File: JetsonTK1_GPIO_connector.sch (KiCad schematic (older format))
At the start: 3 parts

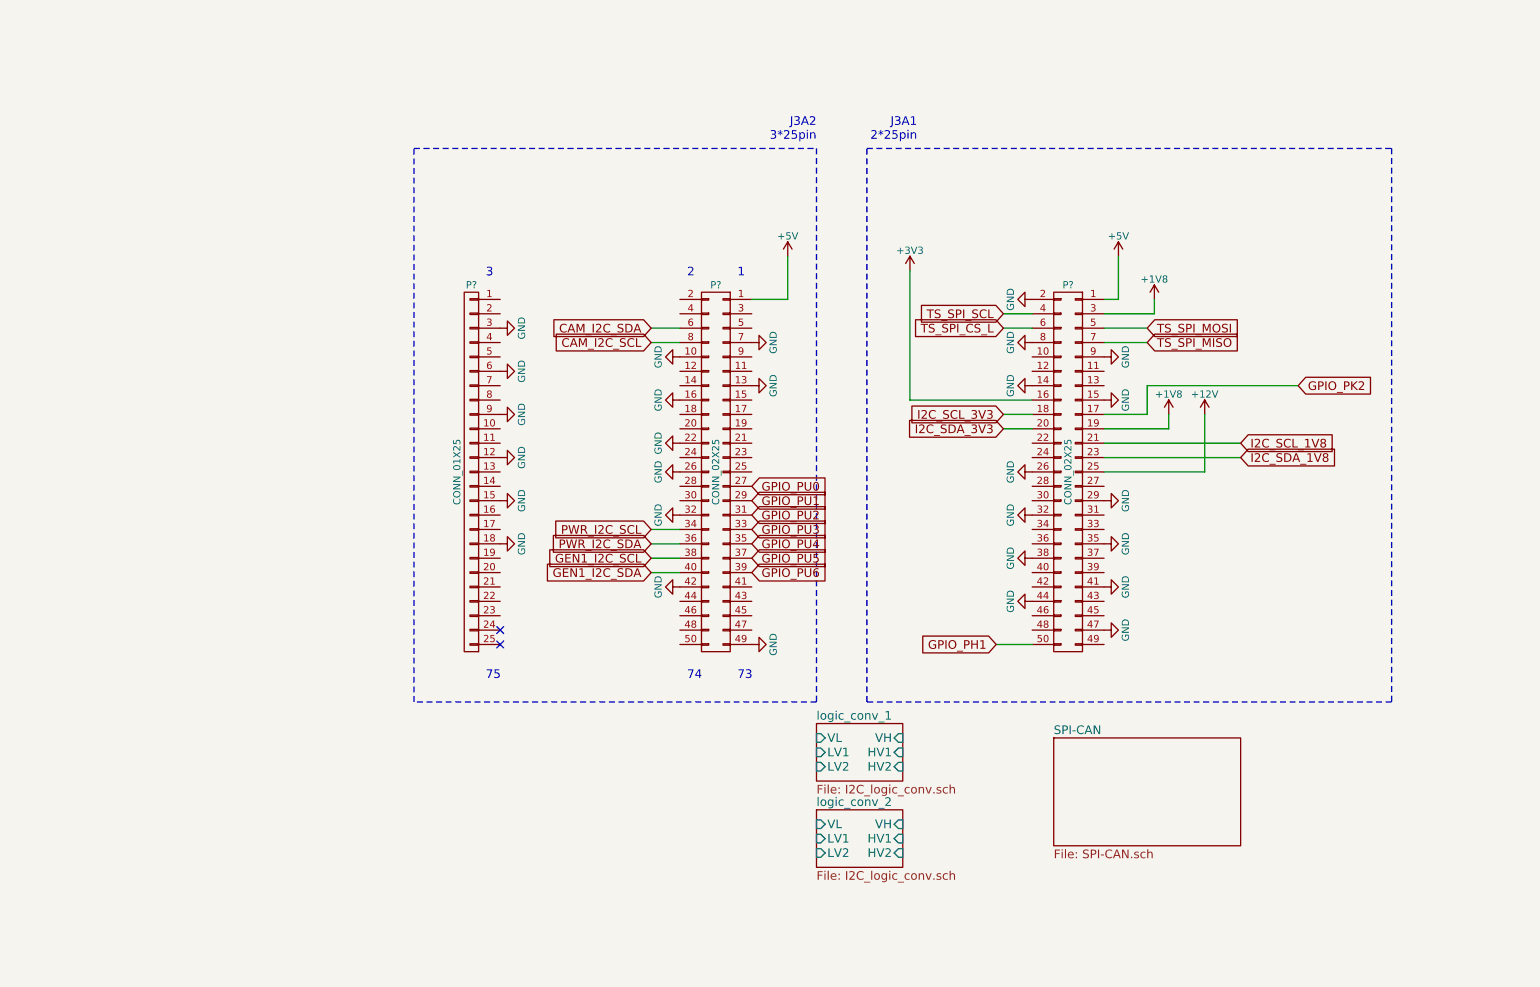
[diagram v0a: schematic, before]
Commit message: IC追加
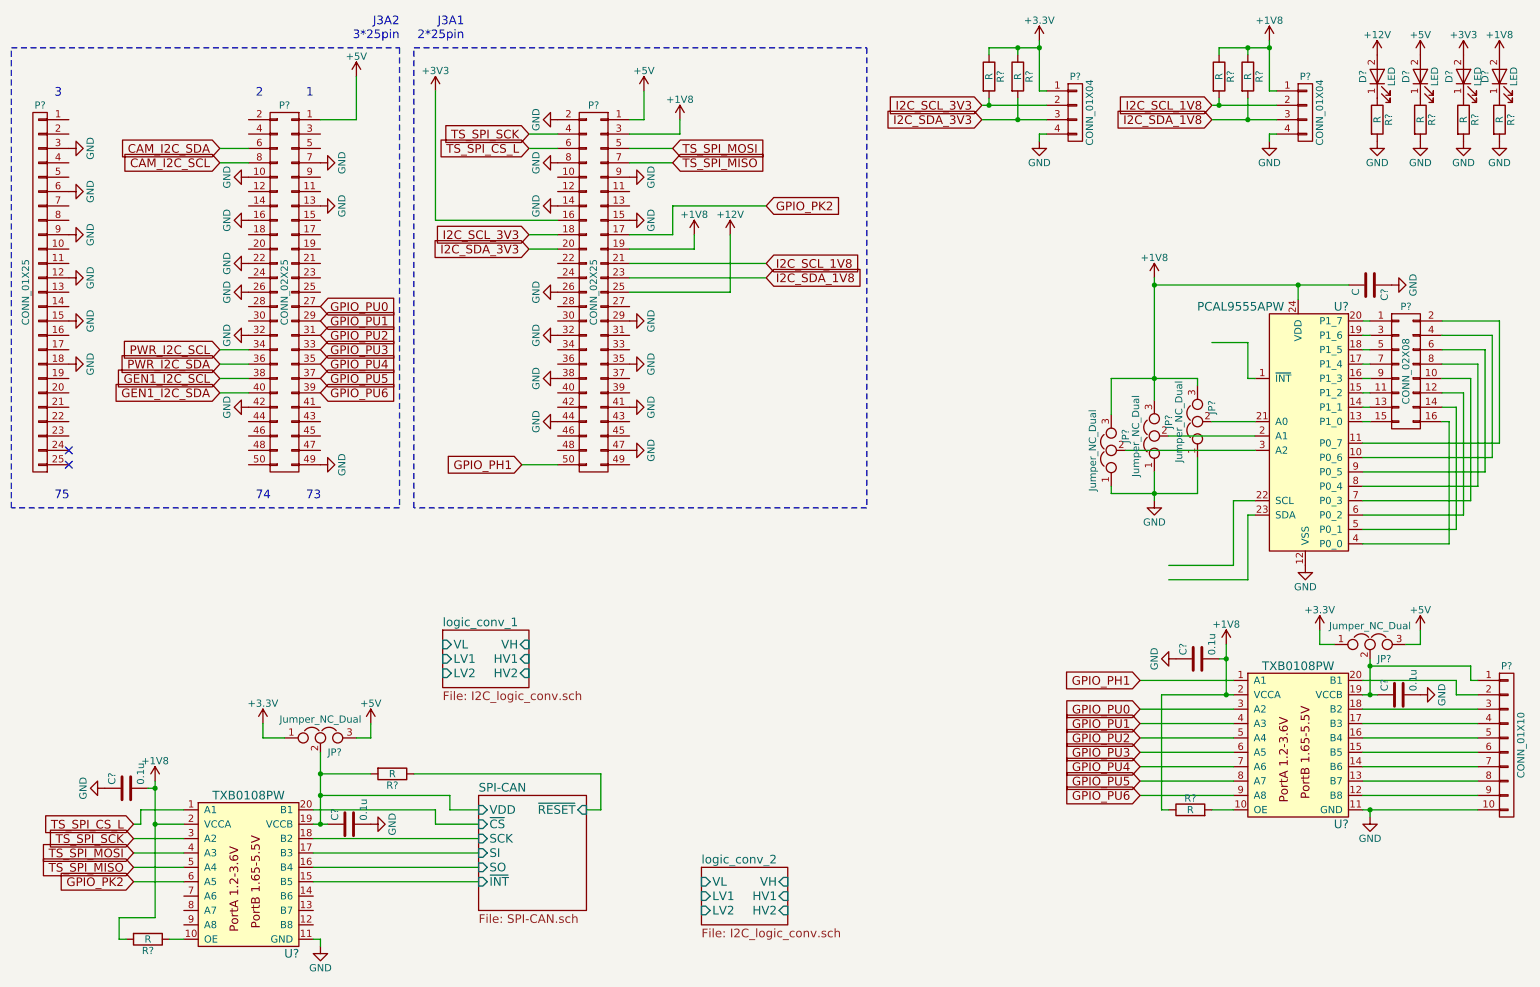
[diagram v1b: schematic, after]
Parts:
- added C? (x4): 0.1u, symbol C
- added C?: C, symbol C
- added D? (x4): LED, symbol LED
- added JP? (x5): Jumper_NC_Dual, symbol Jumper_NC_Dual
- added P? (x2): CONN_01X04, symbol CONN_01X04
- added P?: CONN_02X08, symbol CONN_02X08
- added P?: CONN_01X10, symbol CONN_01X10
- added R? (x11): R, symbol R
- added U? (x2): TXB0108PW, Housings_SSOP:TSSOP-20_4.4x6.5mm_Pitch0.65mm, symbol TXB0108PW
- added U?: PCAL9555APW, Housings_SSOP:TSSOP-24_4.4x7.8mm_Pitch0.65mm, symbol PCAL9555APW
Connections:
- net +12V: now also D?.2 (A)
- net +1V8: now also C?.2, C?.2, C?.2, D?.2 (A), JP?.3, JP?.3, JP?.3, P?.1 (P1), R?.1, R?.1, R?.1, R?.2, U?.2 (VCCA), U?.2 (VCCA), U?.24 (VDD)
- net +3V3: now also D?.2 (A), JP?.1, JP?.1, P?.1 (P1), R?.1, R?.1
- net +5V: now also D?.2 (A), JP?.3, JP?.3
- net GND: now also C?.1, C?.1, C?.1, C?.2, C?.2, JP?.1, JP?.1, JP?.1, P?.10 (P10), P?.4 (P4), P?.4 (P4), R?.2, R?.2, R?.2, R?.2, U?.11 (GND), U?.11 (GND), U?.12 (VSS)
- net GPIO_PH1: now also U?.1 (A1)
- net GPIO_PK2: now also U?.6 (A5)
- net GPIO_PU0: now also U?.3 (A2)
- net GPIO_PU1: now also U?.4 (A3)
- net GPIO_PU2: now also U?.5 (A4)
- net GPIO_PU3: now also U?.6 (A5)
- net GPIO_PU4: now also U?.7 (A6)
- net GPIO_PU5: now also U?.8 (A7)
- net GPIO_PU6: now also U?.9 (A8)
- net I2C_SCL_1V8: now also P?.2 (P2), R?.2
- net I2C_SCL_3V3: now also P?.2 (P2), R?.2
- net I2C_SDA_1V8: now also P?.3 (P3), R?.2
- net I2C_SDA_3V3: now also P?.3 (P3), R?.2
- net TS_SPI_CS_L: now also U?.1 (A1)
- net TS_SPI_MISO: now also U?.5 (A4)
- net TS_SPI_MOSI: now also U?.4 (A3)
- net TS_SPI_SCL renamed TS_SPI_SCK
- net TS_SPI_SCK: now also U?.3 (A2)
- new net: R?.1, U?.10 (OE)
- new net: P?.4 (P4), U?.10 (P0_6)
- new net: P?.2 (P2), U?.11 (P0_7)
- new net: P?.15 (P15), U?.13 (P1_0)
- new net: P?.13 (P13), U?.14 (P1_1)
- new net: P?.11 (P11), U?.15 (P1_2)
- new net: P?.9 (P9), U?.16 (P1_3)
- new net: P?.7 (P7), U?.17 (P1_4)
- new net: P?.5 (P5), U?.18 (P1_5)
- new net: P?.3 (P3), U?.19 (P1_6)
- new net: JP?.2, U?.2 (A1)
- new net: P?.1 (P1), U?.20 (P1_7)
- new net: JP?.2, U?.21 (A0)
- new net: JP?.2, U?.3 (A2)
- new net: P?.16 (P16), U?.4 (P0_0)
- new net: P?.14 (P14), U?.5 (P0_1)
- new net: P?.12 (P12), U?.6 (P0_2)
- new net: P?.10 (P10), U?.7 (P0_3)
- new net: P?.8 (P8), U?.8 (P0_4)
- new net: P?.6 (P6), U?.9 (P0_5)
- new net: D?.1 (K), R?.1 (x4)
- new net: R?.2, U?.10 (OE)
- new net: P?.9 (P9), U?.12 (B8)
- new net: P?.8 (P8), U?.13 (B7)
- new net: P?.7 (P7), U?.14 (B6)
- new net: P?.6 (P6), U?.15 (B5)
- new net: P?.5 (P5), U?.16 (B4)
- new net: P?.4 (P4), U?.17 (B3)
- new net: P?.3 (P3), U?.18 (B2)
- new net: C?.1, JP?.2, P?.1 (P1), U?.19 (VCCB)
- new net: P?.2 (P2), U?.20 (B1)
- new net SPI-CAN/SCK: U?.18 (B2)
- new net SPI-CAN/SI: U?.17 (B3)
- new net SPI-CAN/SO: U?.16 (B4)
- new net SPI-CAN/VDD: C?.1, JP?.2, R?.2, U?.19 (VCCB)
- new net SPI-CAN/~CS: U?.20 (B1)
- new net SPI-CAN/~INT: U?.15 (B5)
- new net SPI-CAN/~RESET: R?.1
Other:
- moved on the sheet: P?
